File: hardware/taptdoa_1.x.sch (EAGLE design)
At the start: 60 parts, among them J1 105017-0001, U1 AP2112K-3.3TRG1, U2 STM32F103RBT6, Y1 8MHz

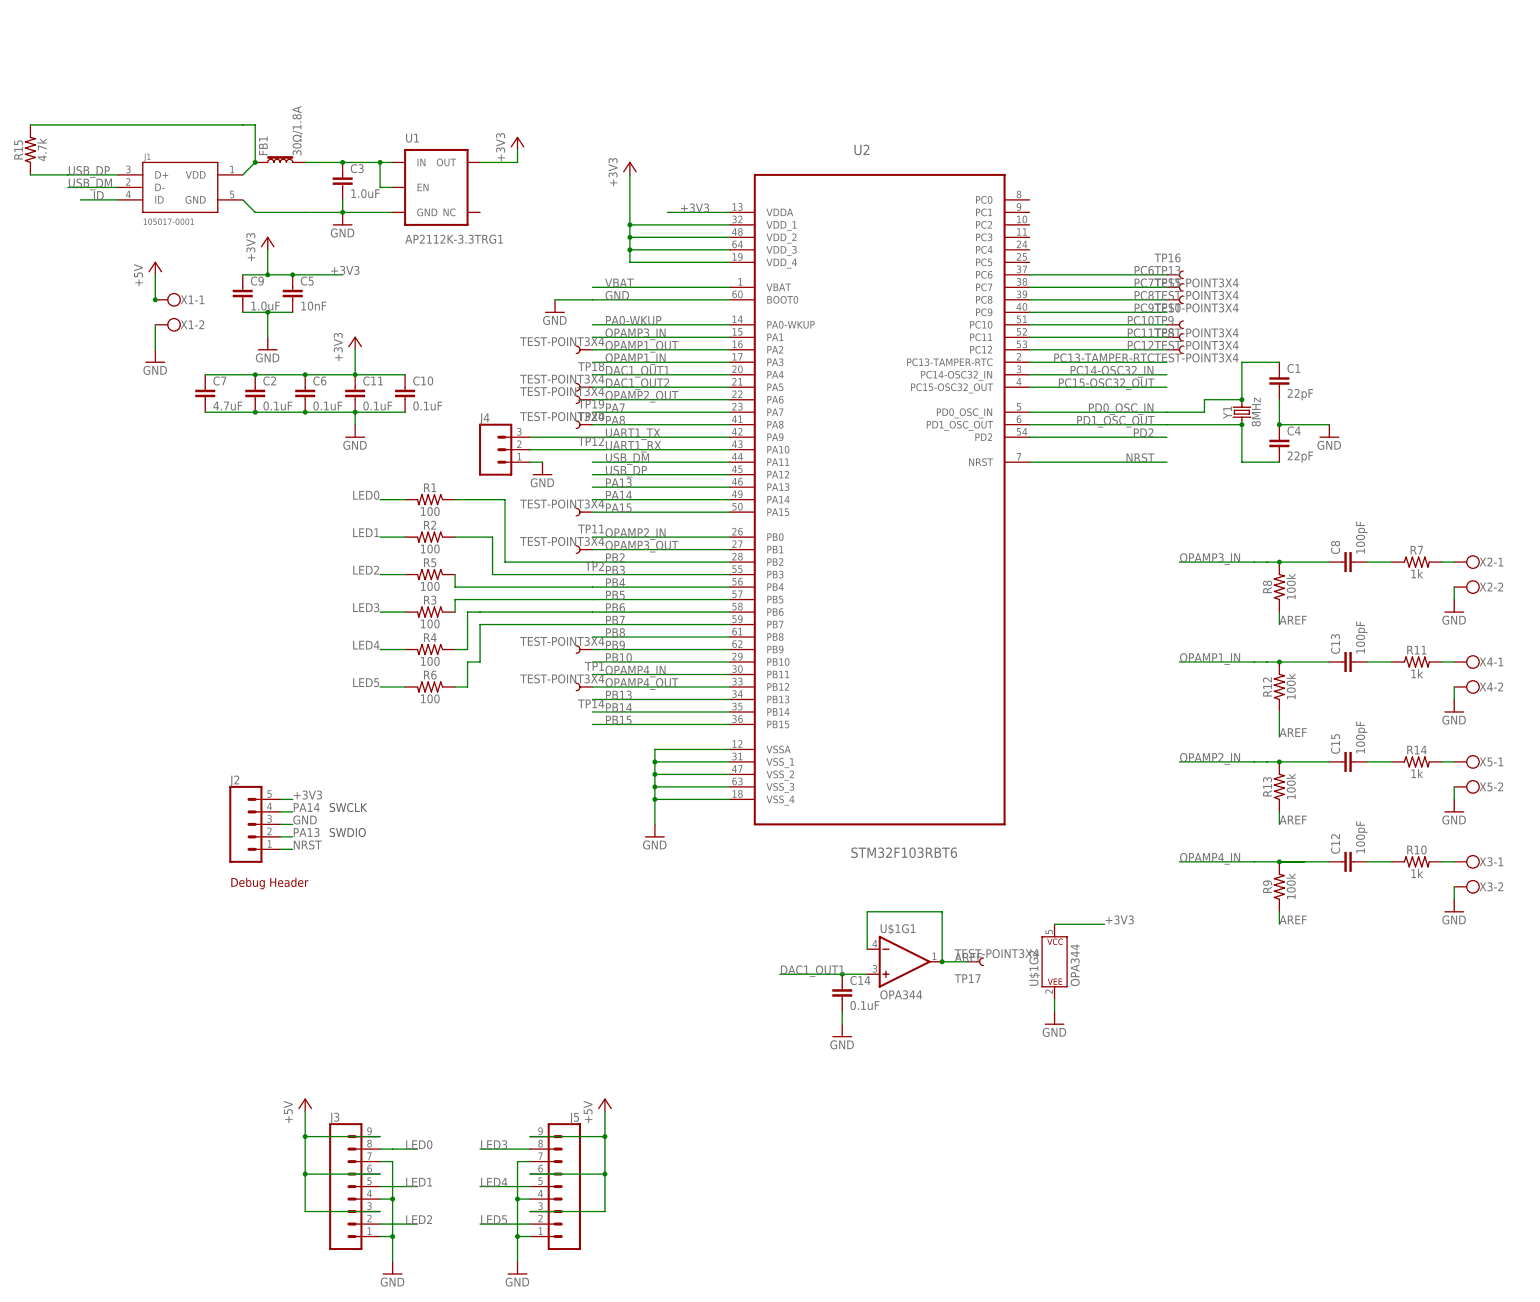
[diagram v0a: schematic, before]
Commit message: re layout board
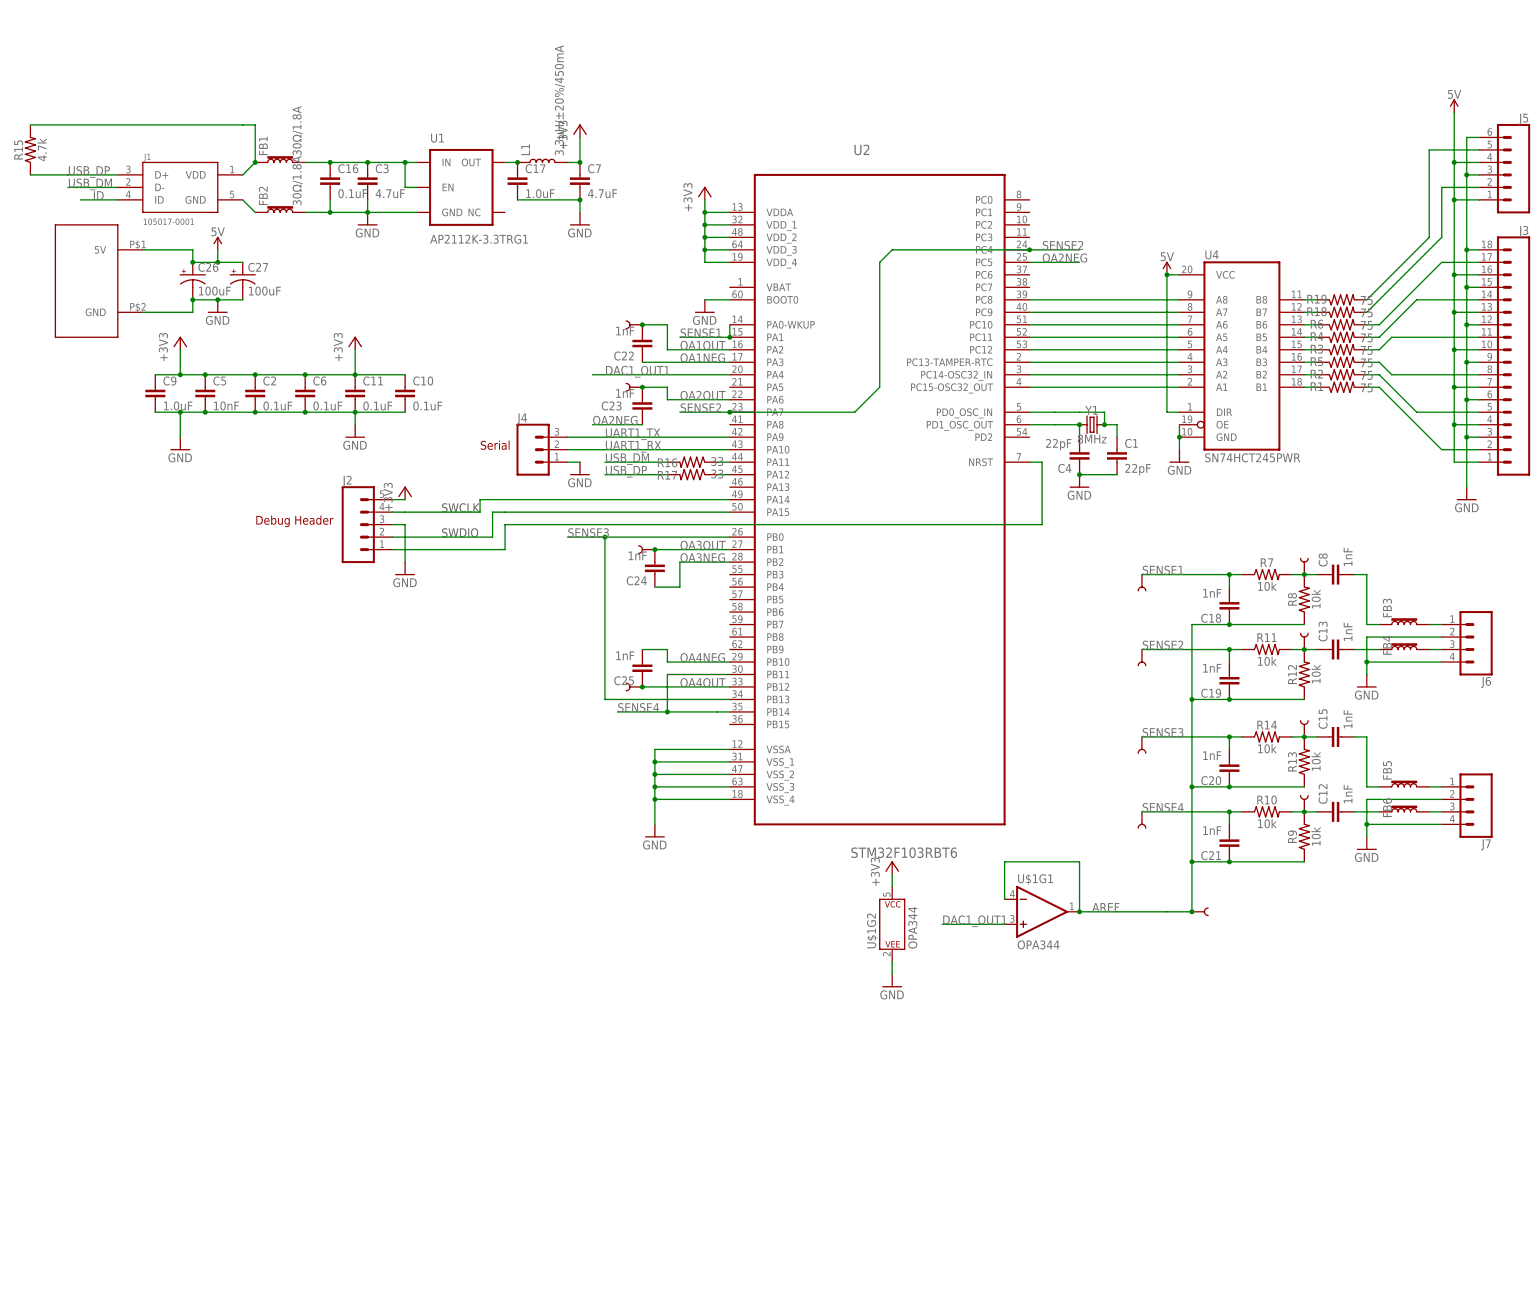
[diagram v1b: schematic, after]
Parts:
- removed C14: 0.1uF, SparkFun-Capacitors:0.1UF-0603-25V-5%
- removed TP13, TP14, TP15, TP16, TP18, TP19, TP20: TEST-POINT3X4, SparkFun-Connectors:TEST-POINT3X4
- removed X1, X2, X3, X4, X5: (no value), con-wago-500:W237-102
- added C16: 0.1uF, SparkFun-Capacitors:0.1UF-0603-25V-5%
- added C17: 1.0uF, SparkFun-Capacitors:1.0UF-0603-16V-10%
- added C18, C19, C20, C21, C22, C23, C24, C25: 1nF, SparkFun-Capacitors:1.0UF-0603-16V-10%
- added C26, C27: 100uF, SparkFun-Capacitors:100UF-POLAR-25V-20%(ELEC)
- added FB2, FB3, FB4, FB5, FB6: 30Ω/1.8A, SparkFun-Coils:FERRITE_BEAD-0603
- added J6, J7: (no value), SparkFun-Connectors:CONN_04LOCK_LONGPADS
- added L1: 3.3µH/±20%/450mA, SparkFun-Coils:INDUCTOR-0805-3.3UH
- added R16, R17: 33, SparkFun-Resistors:100OHM-0603-1/4W-5%
- added R18, R19: 75, SparkFun-Resistors:100OHM-0603-1/4W-5%
- added TP3, TP4, TP5, TP6, TP7: TEST-POINT3X4, SparkFun-Connectors:TEST-POINT3X4
- added U$2: XT30XT30_THRUHOLE, XT30Male:XT30XT30_THRUHOLE
- added U4: SN74HCT245PWR, scanlime:74245PW
- C12, C13, C15, C8: value 100pF -> 1nF
- C3: value 1.0uF -> 4.7uF
- J3: device SparkFun-Connectors:CONN_09LOCK-LONGPADS -> SparkFun-Connectors:CONN_18
- J5: device SparkFun-Connectors:CONN_09LOCK-LONGPADS -> SparkFun-Connectors:CONN_06LOCK
- R1, R2, R3, R4, R5, R6: value 100 -> 75
- R10, R11, R14, R7: value 1k -> 10k
- R12, R13, R8, R9: value 100k -> 10k
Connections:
- removed net +5V: J3.3, J3.6, J3.9, J5.3, J5.6, J5.9, X1-1.KL
- removed net DAC1_OUT2: TP19.1, U2.PA5
- removed net N$1: R7.2, X2-1.KL
- removed net N$3: R11.2, X4-1.KL
- removed net N$5: R14.2, X5-1.KL
- removed net N$7: C12.2, R10.1
- removed net OPAMP1_IN: C13.1, R12.2, U2.PA3
- removed net OPAMP1_OUT: TP18.1, U2.PA2
- removed net OPAMP2_IN: C15.1, R13.2, U2.PB0
- removed net OPAMP2_OUT: TP20.1, U2.PA6
- removed net OPAMP3_IN: C8.1, R8.2, U2.PA1
- removed net OPAMP3_OUT: TP2.1, U2.PB1
- removed net OPAMP4_IN: C12.1, R9.2, U2.PB11
- removed net OPAMP4_OUT: TP14.1, U2.PB12
- removed net PA0-WKUP: U2.PA0-WKUP
- removed net PA15: TP11.1, U2.PA15
- removed net PA7: U2.PA7
- removed net PA8: TP12.1, U2.PA8
- removed net PB10: U2.PB10
- removed net PB13: U2.PB13
- removed net PB14: U2.PB14
- removed net PB15: U2.PB15
- removed net PB2: R1.1, U2.PB2
- removed net PB3: R2.1, U2.PB3
- removed net PB4: R5.1, U2.PB4
- removed net PB5: R3.1, U2.PB5
- removed net PB6: R4.1, U2.PB6
- removed net PB7: R6.1, U2.PB7
- removed net PB8: U2.PB8
- removed net PB9: TP1.1, U2.PB9
- removed net PC10: TP10.1, U2.PC10
- removed net PC11: TP9.1, U2.PC11
- removed net PC12: TP8.1, U2.PC12
- removed net PC13-TAMPER-RTC: U2.PC13-TAMPER-RTC
- removed net PC14-OSC32_IN: U2.PC14-OSC32_IN
- removed net PC15-OSC32_OUT: U2.PC15-OSC32_OUT
- removed net PC6: TP16.1, U2.PC6
- removed net PC7: TP13.1, U2.PC7
- removed net PC8: TP15.1, U2.PC8
- removed net PC9: U2.PC9
- removed net PD2: U2.PD2
- removed net VBAT: U2.VBAT
- new net 5V: C26.+, C27.+, J3.1, J3.10, J3.13, J3.16, J3.4, J3.7, J5.1, J5.4, U$2.5V, U4.DIR, U4.VCC
- new net HP1: C8.1, R7.2, R8.2, TP9.1
- new net HP2: C13.1, R11.2, R12.2, TP10.1
- new net HP3: C15.1, R13.2, R14.2, TP11.1
- new net HP4: C12.1, R10.2, R9.2, TP12.1
- new net N$10: R17.1, U2.PA12
- new net N$11: FB2.1, J1.GND
- new net N$12: C17.1, L1.1, U1.OUT
- new net N$13: R1.1, U4.B1
- new net N$14: R2.1, U4.B2
- new net N$15: R5.1, U4.B3
- new net N$16: R3.1, U4.B4
- new net N$17: R4.1, U4.B5
- new net N$18: R6.1, U4.B6
- new net N$19: C8.2, FB3.1
- new net N$20: C15.2, FB5.1
- new net N$21: C13.2, FB4.1
- new net N$22: U2.PC12, U4.A4
- new net N$23: C12.2, FB6.1
- new net N$24: U2.PC13-TAMPER-RTC, U4.A3
- new net N$25: U2.PC14-OSC32_IN, U4.A2
- new net N$26: U2.PC15-OSC32_OUT, U4.A1
- new net N$27: R18.1, U4.B7
- new net N$28: R19.1, U4.B8
- new net N$29: J5.2, R18.2
- new net N$30: J5.5, R19.2
- new net N$31: FB3.2, J6.1
- new net N$32: FB5.2, J7.1
- new net N$33: FB6.2, J7.3
- new net N$34: FB4.2, J6.3
- new net N$9: R16.1, U2.PA11
- new net OA1NEG: C22.1, U2.PA3
- new net OA1OUT: C22.2, TP4.1, U2.PA2
- new net OA2NEG: C23.1, U2.PC5
- new net OA2OUT: C23.2, TP3.1, U2.PA6
- new net OA3NEG: C24.1, U2.PB2
- new net OA3OUT: C24.2, TP1.1, U2.PB1
- new net OA4NEG: C25.2, U2.PB10
- new net OA4OUT: C25.1, TP2.1, U2.PB12
- new net SENSE1: C18.2, R7.1, TP8.1, U2.PA0-WKUP, U2.PA1
- new net SENSE2: C19.2, R11.1, TP7.1, U2.PA7, U2.PC4
- new net SENSE3: C20.2, R14.1, TP6.1, U2.PB0, U2.PB13
- new net SENSE4: C21.2, R10.1, TP5.1, U2.PB11, U2.PB14
- net +3V3: now also L1.2; no longer U1.OUT
- net AREF: now also C18.1, C19.1, C20.1, C21.1
- net DAC1_OUT1: no longer C14.1
- net GND: now also C16.2, C17.2, C26.-, C27.-, FB2.2, J3.12, J3.15, J3.18, J3.3, J3.6, J3.9, J5.3, J5.6, J6.2, J6.4, J7.2, J7.4, U$2.GND, U4.GND, U4.OE; no longer C14.2, J1.GND, J3.1, J3.4, J3.7, J5.1, J5.4, J5.7, X1-2.KL, X2-2.KL, X3-2.KL, X4-2.KL, X5-2.KL
- net LED0: now also J3.2; no longer J3.8
- net LED2: now also J3.8; no longer J3.2
- net LED3: now also J3.11; no longer J5.8
- net LED4: now also J3.14; no longer J5.5
- net LED5: now also J3.17; no longer J5.2
- net N$2: now also U2.PC8, U4.A8; no longer C13.2, R11.1
- net N$4: now also U2.PC9, U4.A7; no longer C15.2, R14.1
- net N$6: now also U2.PC10, U4.A6; no longer R10.2, X3-1.KL
- net N$8: now also U2.PC11, U4.A5; no longer C8.2, R7.1
- net PA13: now also U2.PA15; no longer U2.PA13
- net USB_DM: now also R16.2; no longer U2.PA11
- net USB_DP: now also R17.2; no longer U2.PA12
- net VUSB2: now also C16.1
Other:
- note added: "Serial"
- moved on the sheet: C1, C12, C13, C15, C3, C4, C5, C7, C8, C9, J2, J4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
